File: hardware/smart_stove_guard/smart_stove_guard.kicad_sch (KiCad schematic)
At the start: 29 parts, among them IC1 BS412, J1 12401948E412A, J2 AX-1203D-LF, J3 IO Expansion, U1 ESP32-C6-WROOM-1-N4, U2 MLX90614ESF-AAA-000-TU, U3 AMS1117-3.3

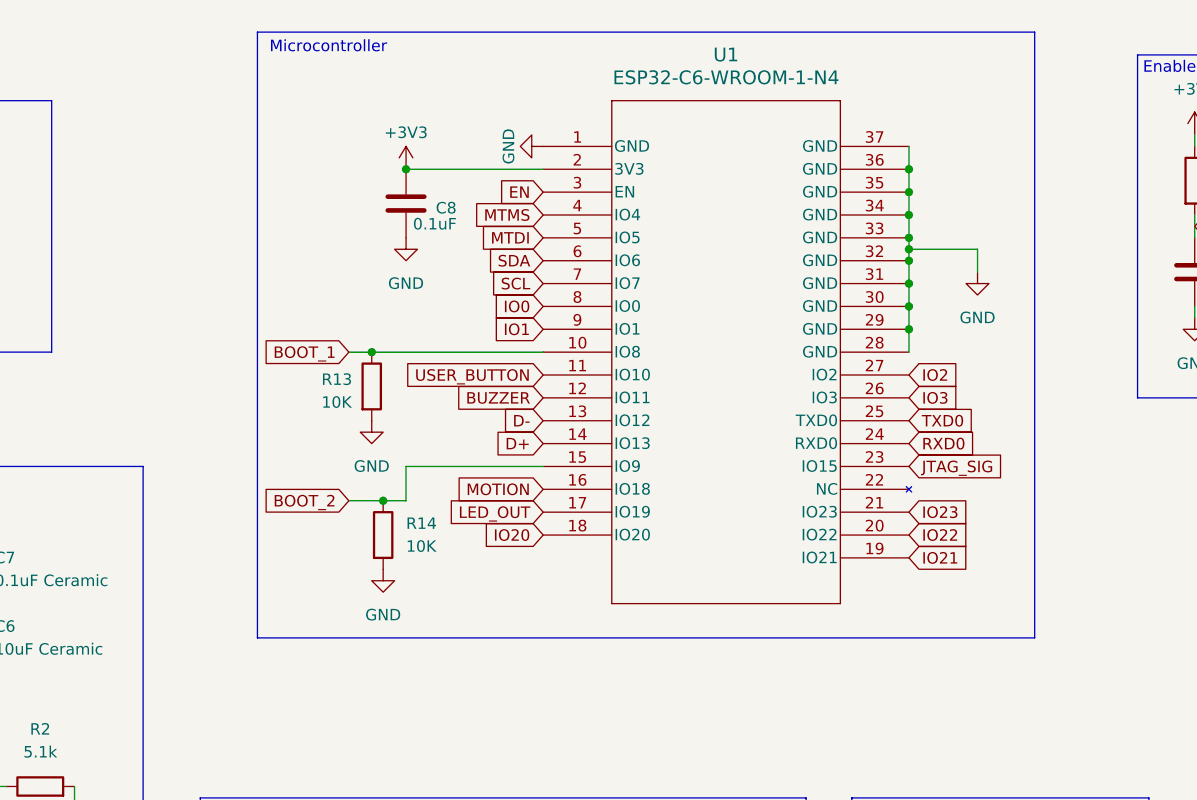
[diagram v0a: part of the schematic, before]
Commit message: minor changes before continuing layout tonight
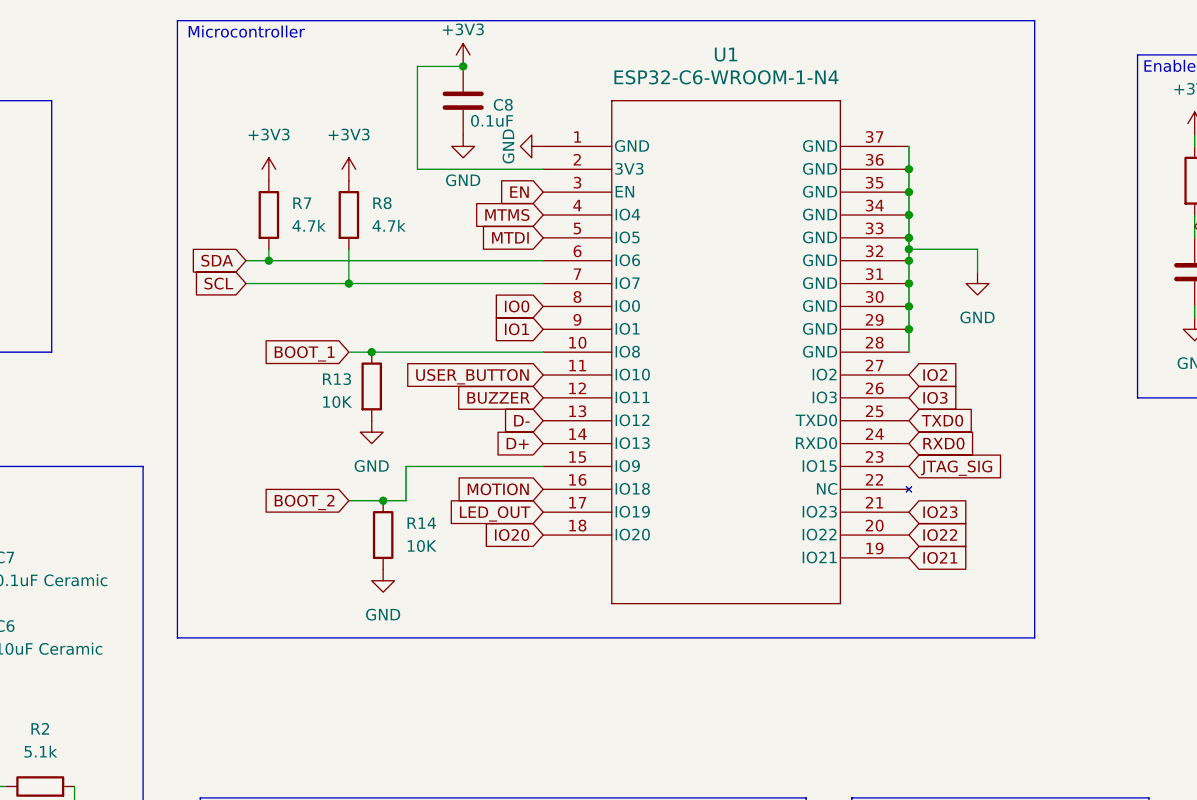
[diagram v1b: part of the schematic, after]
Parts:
- added R7, R8: 4.7k, Resistor_SMD:R_0805_2012Metric, symbol Device:R
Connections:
- net +3V3: now also R7.1, R8.1
- net SCL: now also R8.2
- net SDA: now also R7.2
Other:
- moved on the sheet: C8
